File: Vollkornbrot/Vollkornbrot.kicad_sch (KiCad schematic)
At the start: 29 parts, among them J1 Conn_01x02_Socket, J2 Conn_01x02_Socket, J3 Conn_01x02_Socket, J4 Conn_01x02_Socket, J5 6Pin

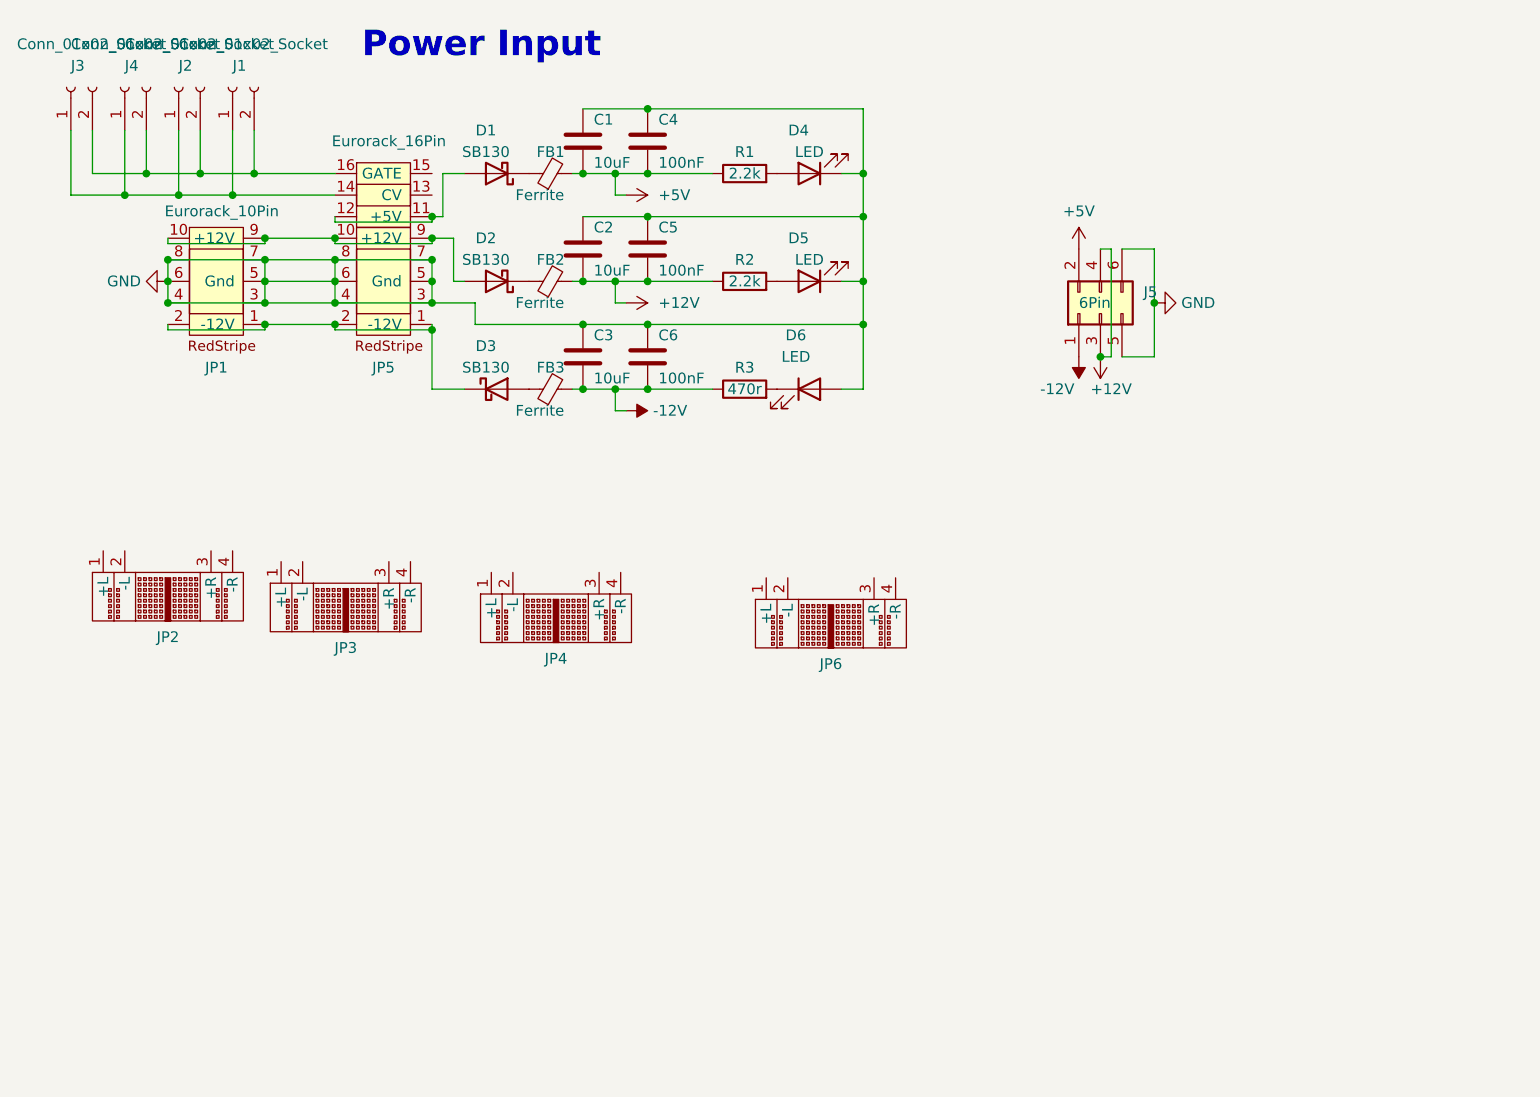
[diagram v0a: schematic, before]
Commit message: Volkornbrot Rev 2 and multiplexter BBF
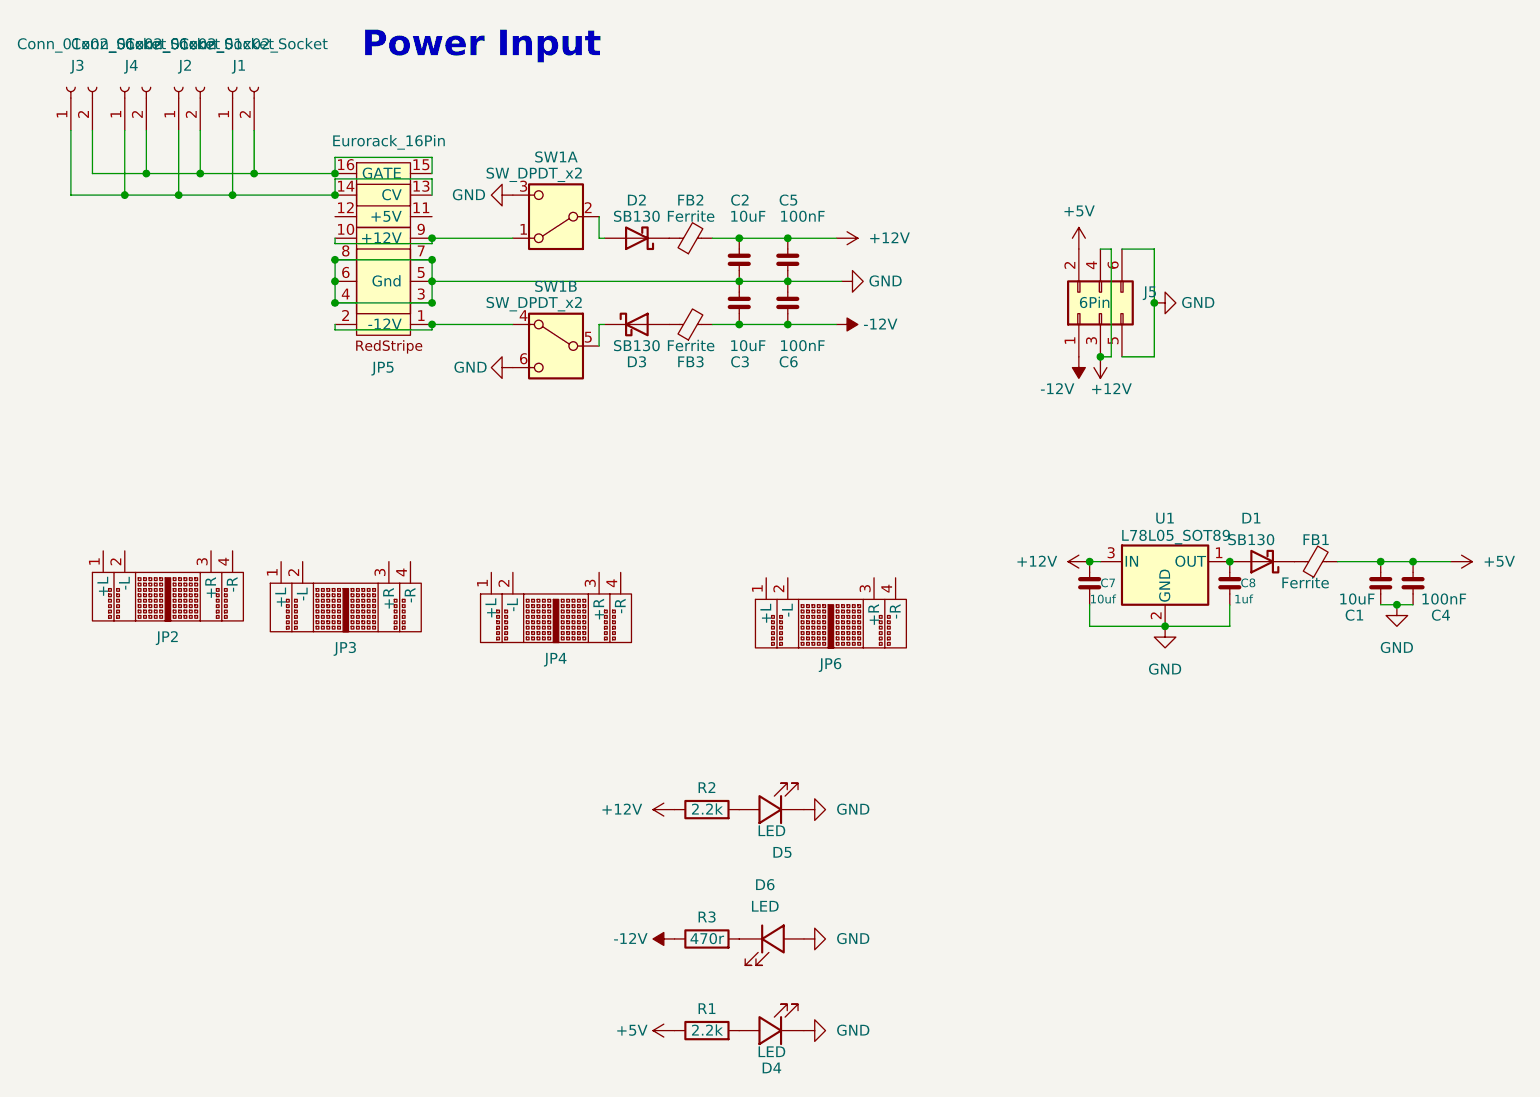
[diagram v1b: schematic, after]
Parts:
- removed JP1: Eurorack_10Pin, Connector_IDC:IDC-Header_2x05_P2.54mm_Vertical_SMD, symbol Schreibmaschine_Interface:Eurorack_10Pin
- added C7: 10uf, Capacitor_SMD:C_1206_3216Metric, symbol Schreibmaschine_Core:C
- added C8: 1uf, Capacitor_SMD:C_1206_3216Metric, symbol Schreibmaschine_Core:C
- added SW1: SW_DPDT_x2, Schreibmaschine_Footprints:SSSS213202, symbol Switch:SW_DPDT_x2
- added U1: L78L05_SOT89, Package_TO_SOT_SMD:SOT-89-3, symbol Regulator_Linear:L78L05_SOT89
- C1, C2, C3, C4, C5, C6: symbol Device:C -> Schreibmaschine_Core:C
- D4, D5, D6: symbol Device:LED -> Schreibmaschine_Interface:LED
- FB1, FB2, FB3: footprint Diode_SMD:D_0603_1608Metric -> Diode_SMD:D_0805_2012Metric
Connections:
- net +12V: now also C7.2, U1.3 (IN)
- net -12V: now also C3.1, C6.1; no longer C3.2, C6.2
- net GND: now also C3.2, C6.2, C7.1, C8.1, SW1.3 (C), SW1.6 (C), U1.2 (GND); no longer C3.1, C6.1
- net at J1.1 (Pin_1), J2.1 (Pin_1), J3.1 (Pin_1)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: now also JP5.13 (CV)
- net at J1.2 (Pin_2), J2.2 (Pin_2), J3.2 (Pin_2)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: now also JP5.15 (GATE)
- net at JP5.10, JP5.9 (+12V): now also SW1.1 (A); no longer D2.2 (A)
- net at JP5.1 (-12V), JP5.2: now also SW1.4 (A); no longer D3.1 (K)
- new net: D2.2 (A), SW1.2 (B)
- new net: C8.2, D1.2 (A), U1.1 (OUT)
- new net: D3.1 (K), SW1.5 (B)
- now unconnected: JP5.11 (+5V), JP5.12
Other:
- moved on the sheet: D1, D2, D3, FB1, FB2, FB3, R1, R2, R3
